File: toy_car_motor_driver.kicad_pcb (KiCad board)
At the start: 2 copper layers, 44 x 35 mm, 15 parts, among them J1 Conn_01x06_Pin, J3 Conn_01x02_Pin, J4 Screw_Terminal_01x02, J5 Screw_Terminal_01x02, J6 Screw_Terminal_01x02, SW1 SW_DIP_x04, U1 L293D

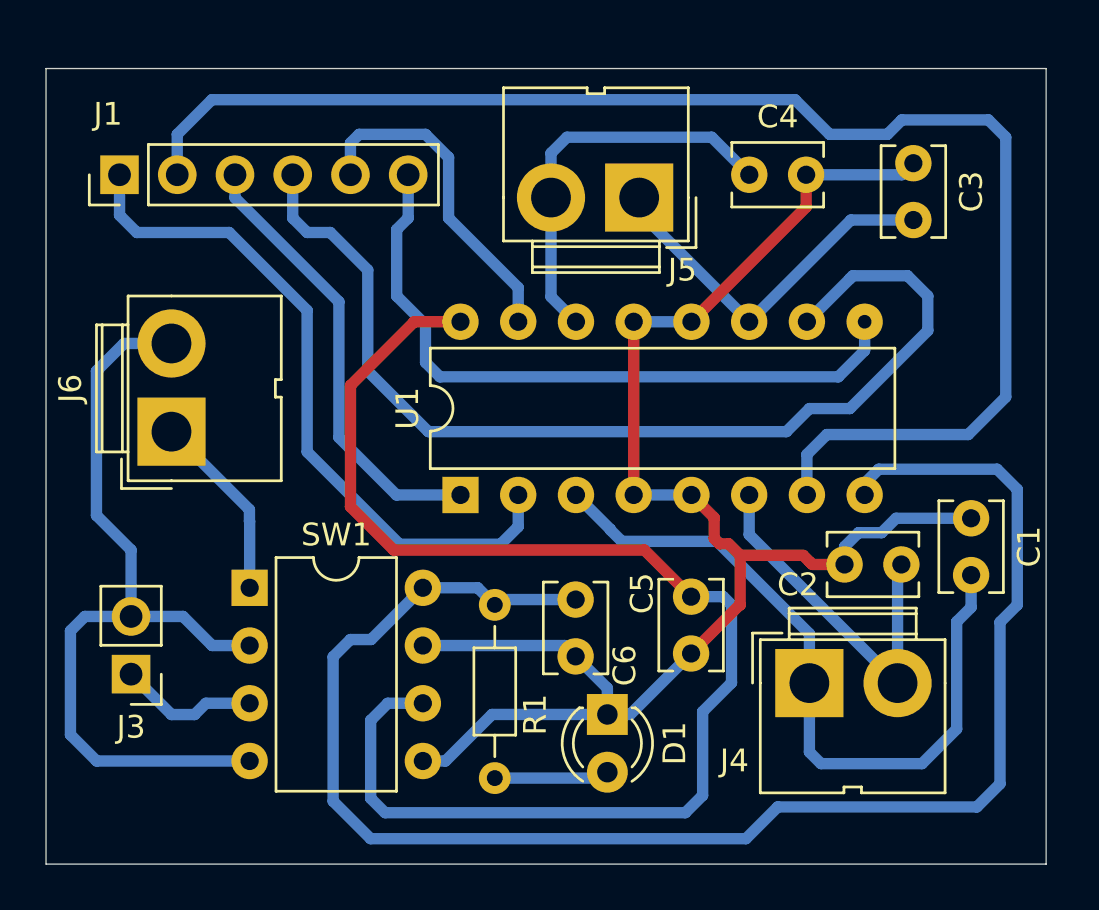
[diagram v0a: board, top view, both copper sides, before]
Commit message: Updated pcb
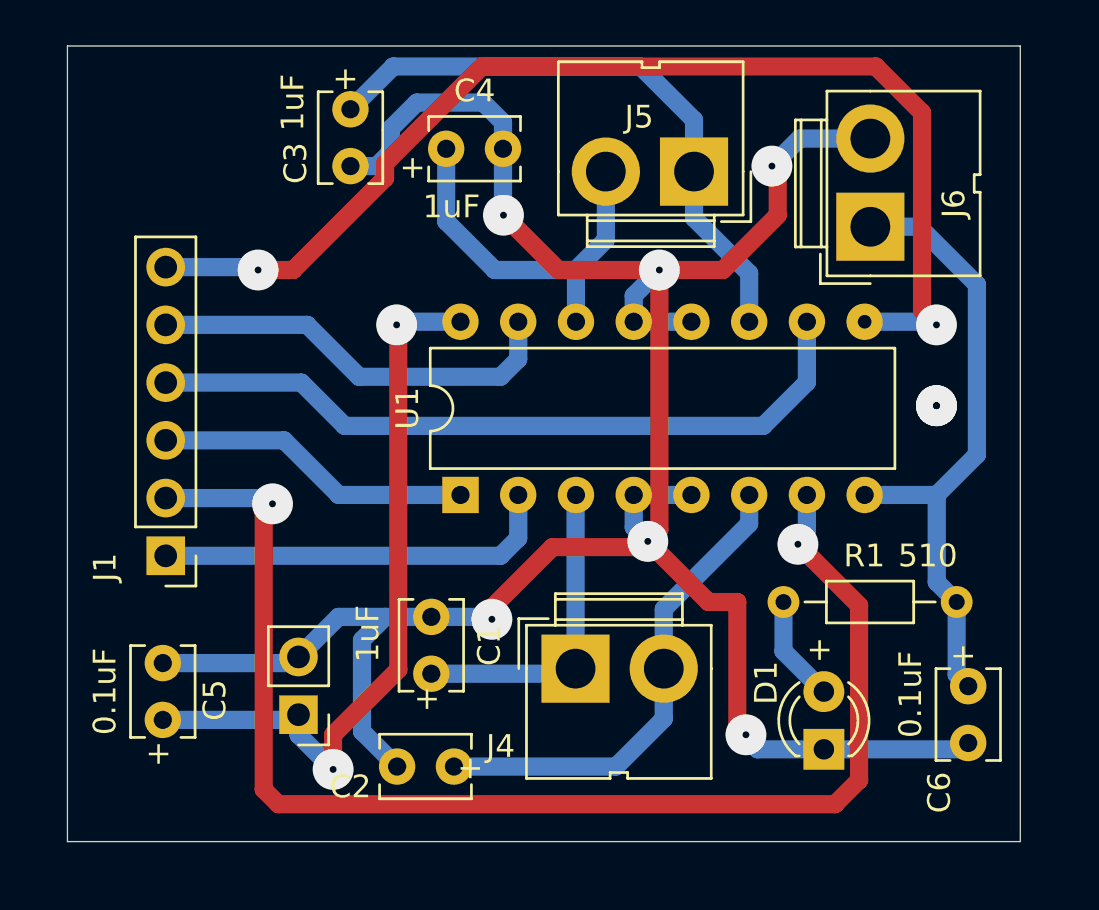
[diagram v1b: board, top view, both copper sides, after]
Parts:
- removed SW1: SW_DIP_x04, Package_DIP:DIP-8_W7.62mm
- moved J6 32.0 mm to (124.3, 65.3)
- moved C3 24.8 mm to (101.5, 62.6), turned to 90 degrees
- moved C1 24.1 mm to (105.0, 82.4)
- moved C5 23.2 mm to (93.2, 84.5), turned to -90 degrees
- moved C2 21.6 mm to (106.0, 89.0)
- moved C6 17.7 mm to (128.7, 85.5)
- moved J1 16.9 mm to (93.3, 79.8), turned to 180 degrees
- moved R1 14.9 mm to (120.5, 81.8), turned to 0 degrees
- moved C4 13.4 mm to (105.7, 61.8)
- moved J4 10.3 mm to (111.4, 84.7)
- moved D1 9.65 mm to (122.3, 88.3), turned to 90 degrees
- moved J3 7.58 mm to (99.2, 86.7)
- moved J5 2.67 mm to (116.6, 62.9)
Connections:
- J3 pad 1: /5V_i -> /5V
- J3 pad 2: /GND_i -> GND
- J6 pad 1: /9V_i -> /9V
- J6 pad 2: /GND_i -> GND
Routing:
- net /9V: track 70.8 -> 27.9 mm
- net GND: track 70.6 -> 109.4 mm, vias 0 -> 6
- net /GND_i: track 36.8 -> 0.00 mm
- net /5V: track 60.0 -> 32.7 mm, vias 0 -> 2
- net /EN_3,4: track 30.3 -> 51.4 mm, vias 0 -> 2
- net /output_1: track 32.4 -> 14.1 mm
- net /input_3A: track 46.2 -> 32.5 mm
- net /input_1A: track 30.7 -> 17.7 mm
- net /output_2: track 16.5 -> 26.8 mm
- net /9V_i: track 8.29 -> 0.00 mm
- net /5V_i: track 6.16 -> 0.00 mm
- net /EN_1,2: track 19.8 -> 14.0 mm
- net /outputr_1: track 16.3 -> 21.5 mm
- net /inputr_2A: track 63.1 -> 58.3 mm, vias 0 -> 2
- net /inputr_4A: track 14.8 -> 18.4 mm
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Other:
- board size 44 x 35 mm -> 41.9 x 35 mm
- board text added: "+"
